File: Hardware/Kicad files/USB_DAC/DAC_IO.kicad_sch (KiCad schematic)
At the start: 12 parts, among them J1 NC3MAH, J10 B4B-PH-K-S, J3 B7B-PH-K-S, J5 Jack-DC, J7 B2B-PH-K-S, J8 NC3MAH, J9 USB4110GFA, U3 IP4234CZ6

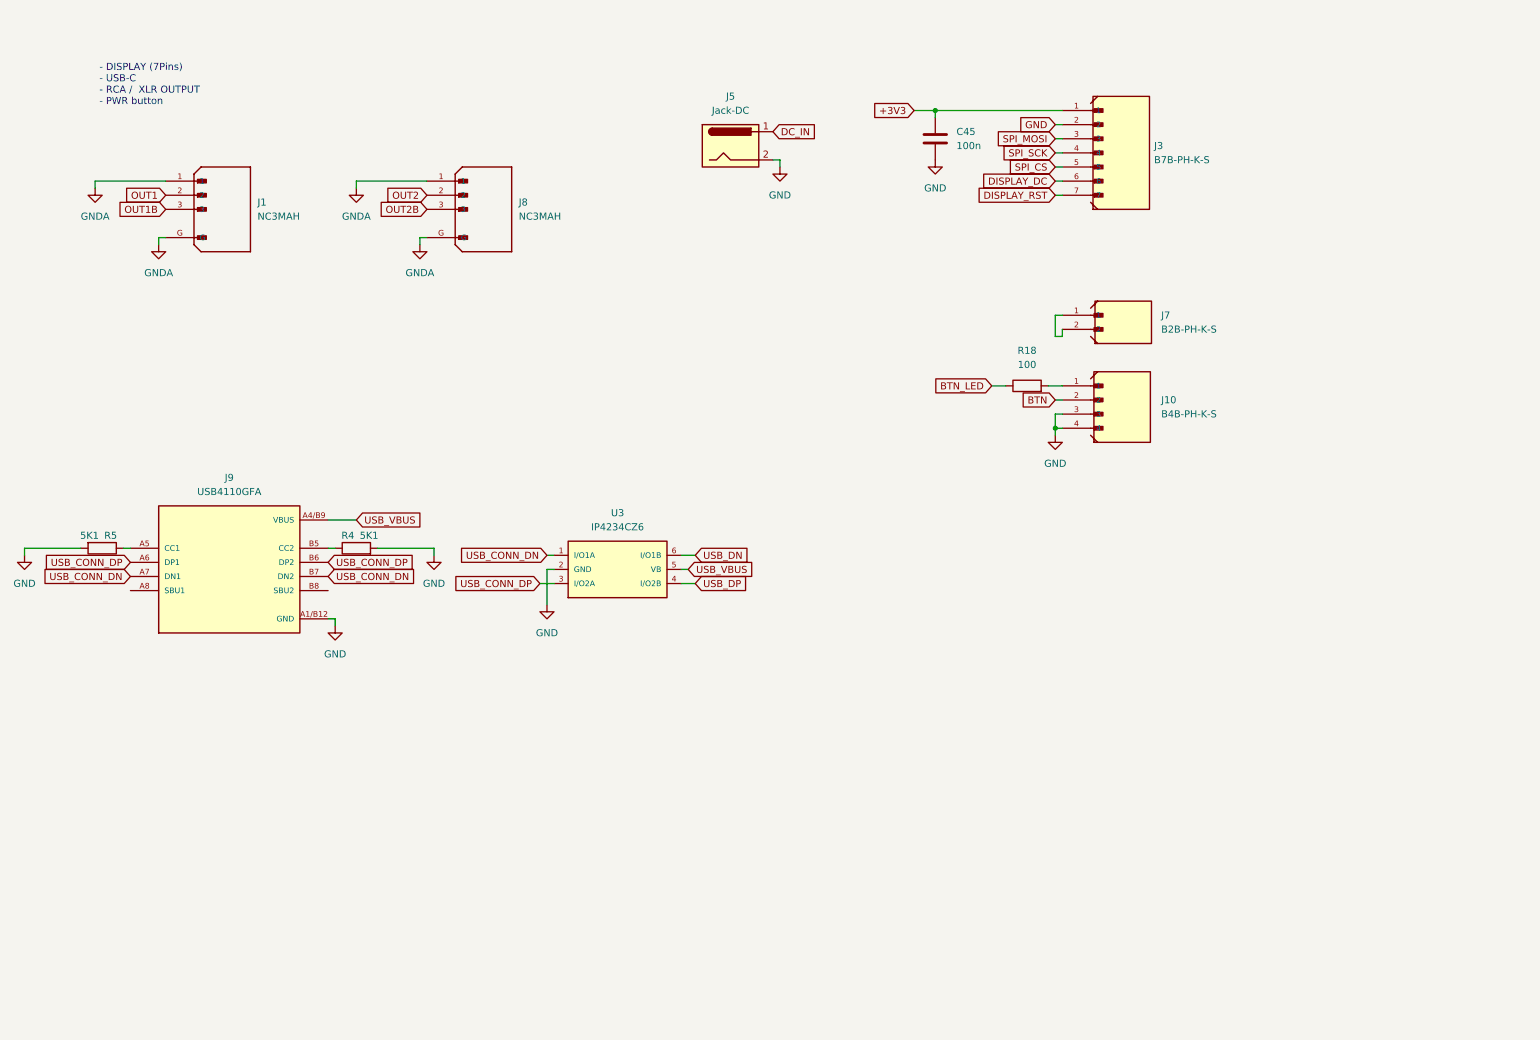
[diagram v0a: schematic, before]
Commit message: Updated PCB and schematics
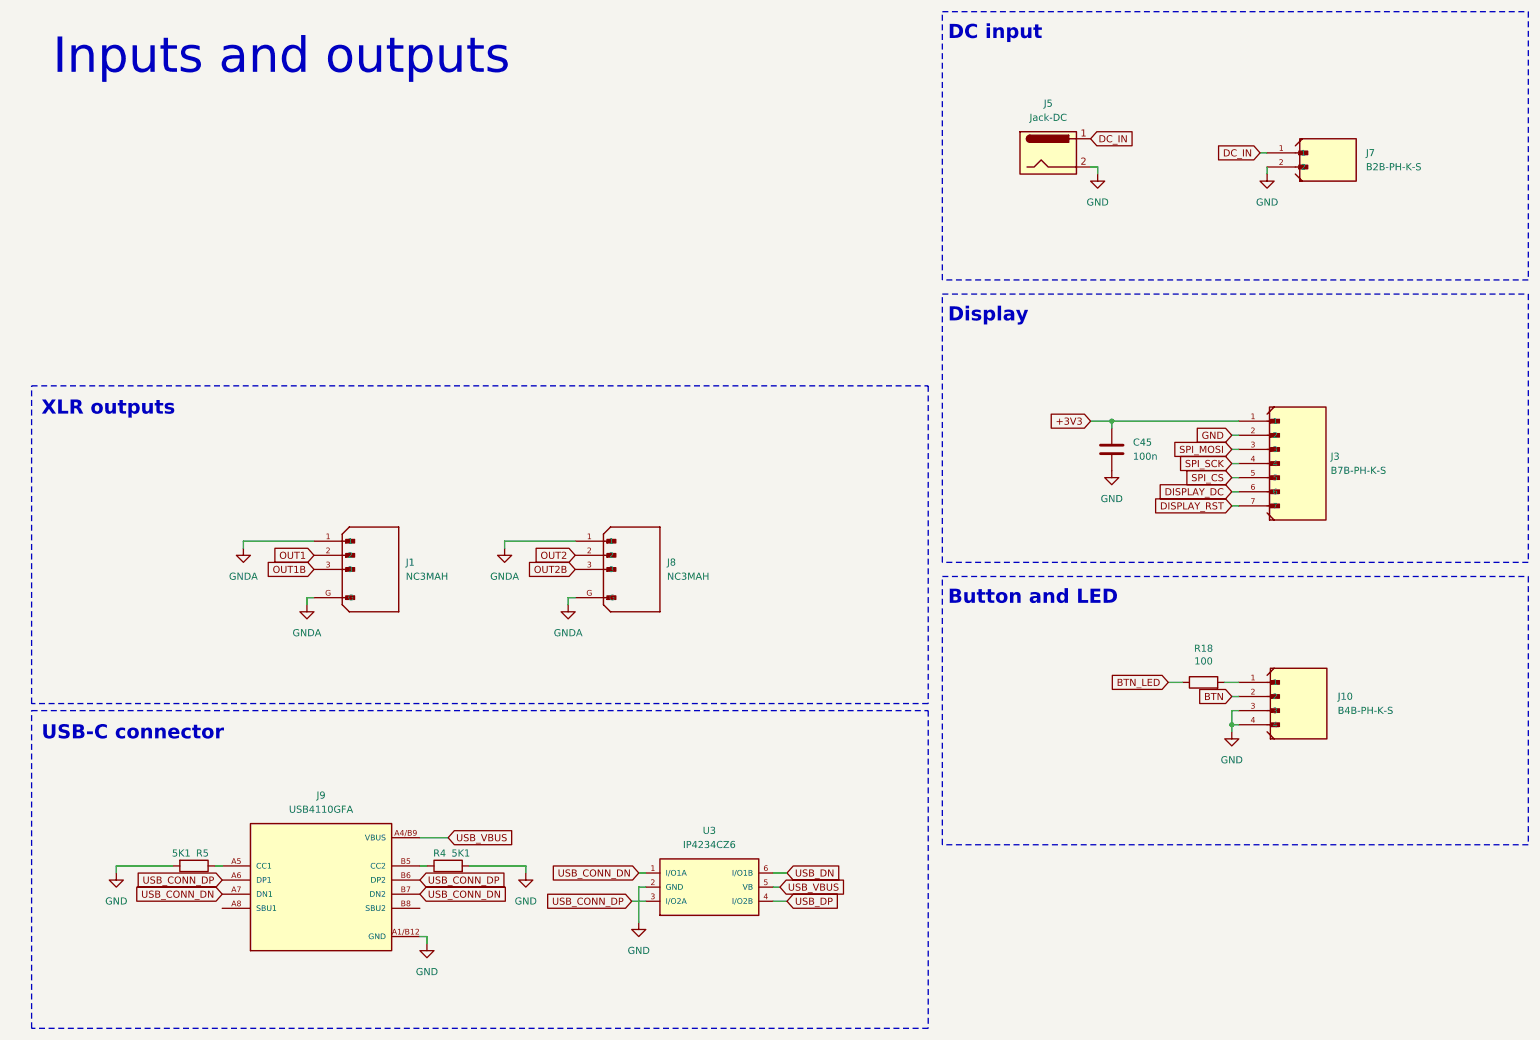
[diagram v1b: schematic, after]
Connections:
- net DC_IN: now also J7.1
- net GND: now also J7.2
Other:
- note added: "Button and LED"
- note added: "DC input"
- note added: "Display"
- note added: "Inputs and outputs"
- note added: "USB-C connector"
- note added: "XLR outputs"
- note removed: "- DISPLAY (7Pins) - USB-C - RCA / XLR OUTPUT - PWR button"
- company: (none) -> Linus Fridlund
- title: (none) -> I/O Sheet
- moved on the sheet: C45, J1, J10, J3, J5, J7, J8, J9, R18, R4, R5, U3
